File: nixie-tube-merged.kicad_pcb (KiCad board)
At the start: 2 copper layers, 99.8 x 97.5 mm, 0 parts

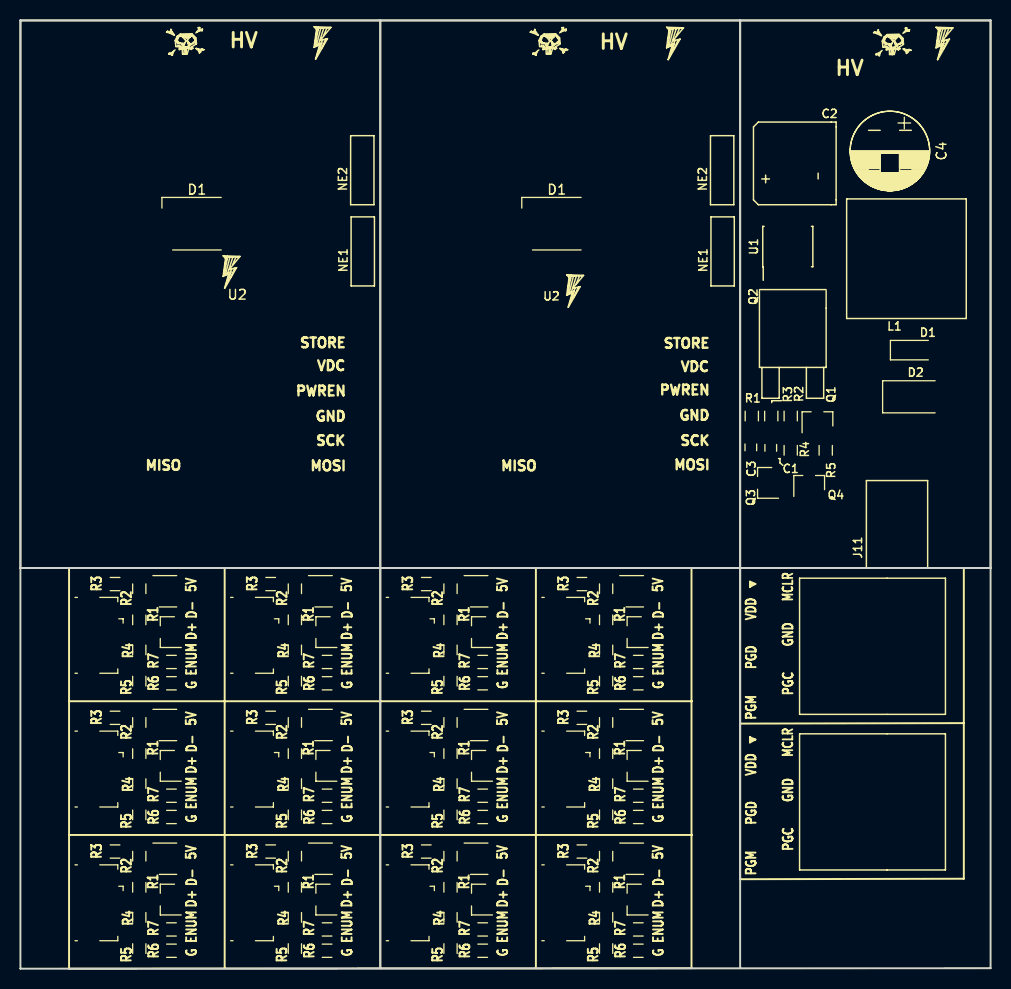
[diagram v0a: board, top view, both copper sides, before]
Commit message: checked all components, modifed some tracks
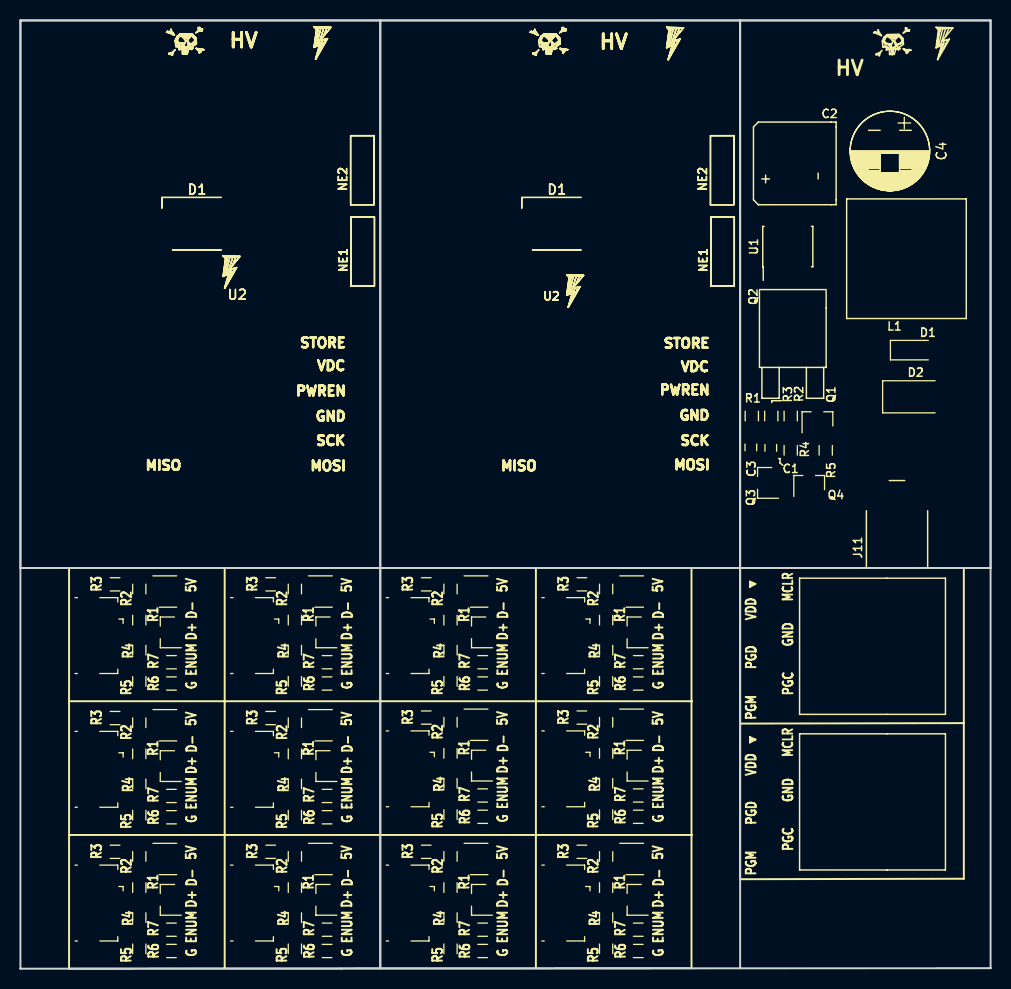
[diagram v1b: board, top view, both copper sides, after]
